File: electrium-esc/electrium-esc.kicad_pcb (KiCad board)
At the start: 2 copper layers, 90 x 60 mm, 181 parts, among them J1 Debug Connector, J2 USB_MICRO, J4 SERVO, J5 Conn_01x04_Male, Q1 IRF3205, Q10 IRF3205, Q11 IRF3205, Q12 IRF3205, Q2 IRF3205, Q3 IRF3205, Q4 IRF3205, Q5 IRF3205, Q6 IRF3205, Q7 IRF3205, Q8 IRF3205, Q9 IRF3205, SW1 SW_SPDT, U1 STM32F407ZGT6, U2 DRV8301DCAR, U3 DRV8301DCAR, U5 NRF24L01_Breakout, Y1 25MHz

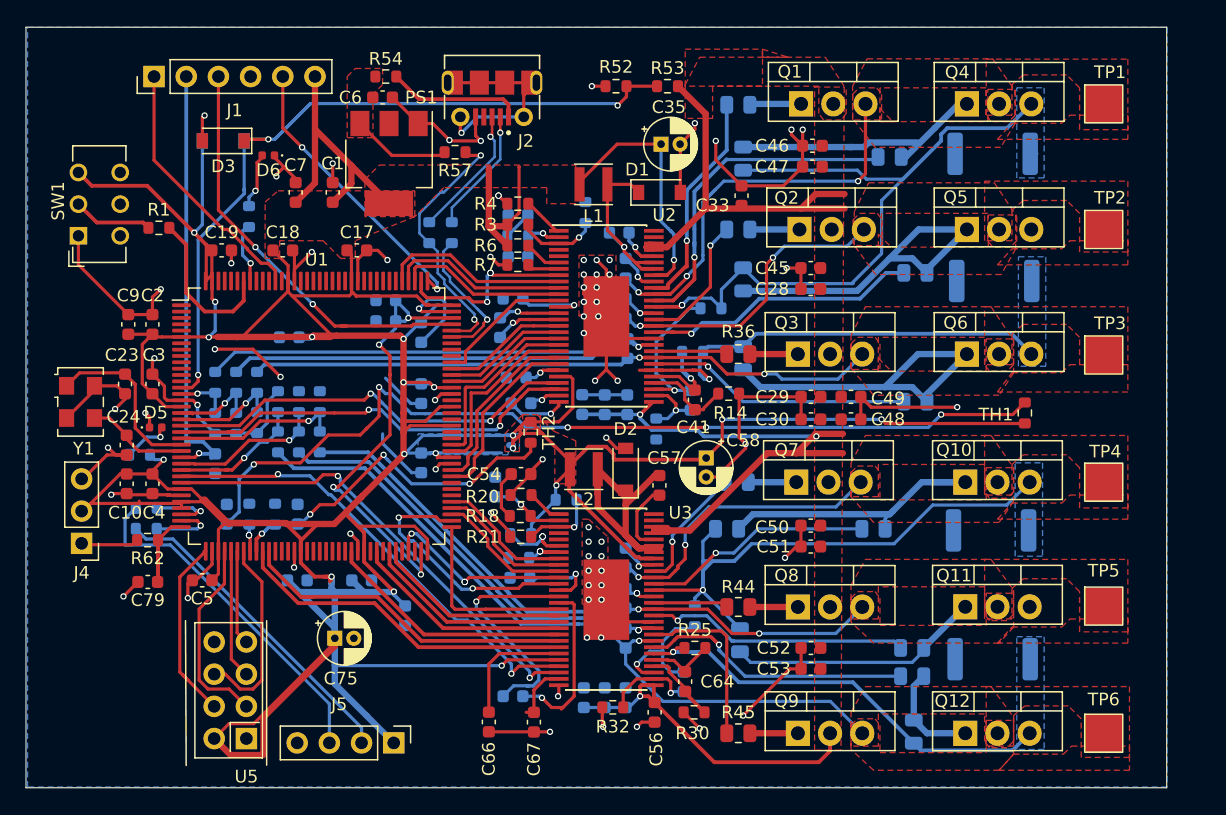
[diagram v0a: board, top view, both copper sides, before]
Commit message: Fix warnings
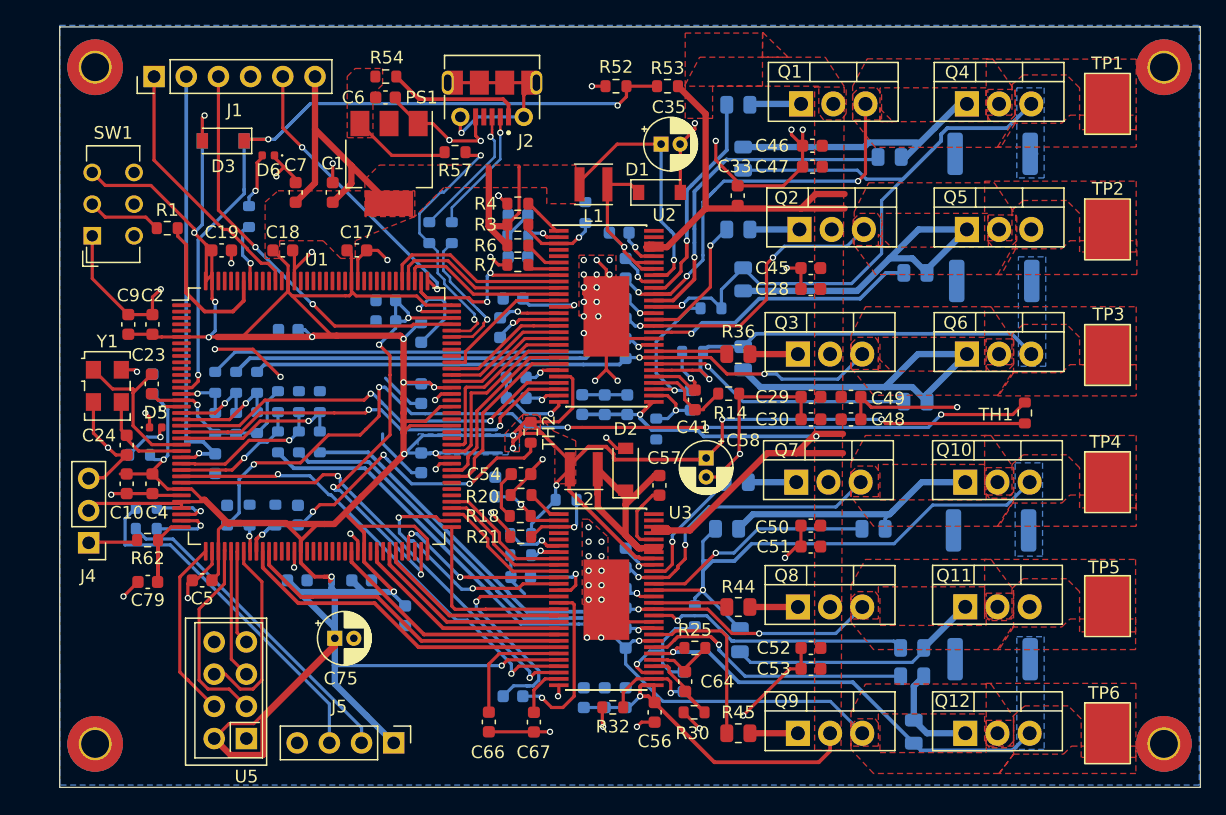
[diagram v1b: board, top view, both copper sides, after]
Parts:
- added REF**: MountingHole_2.2mm_M2_Pad_TopBottom, MountingHole:MountingHole_2.2mm_M2_Pad_TopBottom, F.Cu at (190.8, 102.1)
- added REF**: MountingHole_2.2mm_M2_Pad_TopBottom, MountingHole:MountingHole_2.2mm_M2_Pad_TopBottom, F.Cu at (106.5, 48.7)
- added REF**: MountingHole_2.2mm_M2_Pad_TopBottom, MountingHole:MountingHole_2.2mm_M2_Pad_TopBottom, F.Cu at (190.8, 48.7)
- added asd: MountingHole_2.2mm_M2_Pad_TopBottom, MountingHole:MountingHole_2.2mm_M2_Pad_TopBottom, F.Cu at (106.5, 102.1)
- C3: moved to B.Cu
- moved Y1 2.47 mm to (107.4, 73.8)
- moved C23 2.11 mm to (110.9, 73.7)
- moved SW1 1.09 mm to (106.2, 62.0)
- moved R1 0.66 mm to (112.2, 61.4)
- moved C8 0.59 mm to (121.7, 69.4)
- moved J4 0.56 mm to (106.0, 86.2)
- moved C44 0.56 mm to (139.7, 74.8)
- moved C33 0.30 mm to (157.2, 58.8)
- moved R23 0.25 mm to (140.1, 87.2)
- moved C6 0.23 mm to (129.4, 51.1)
- moved C40 0.15 mm to (148.3, 70.9)
- moved C60 0.08 mm to (140.1, 88.9)
- moved C76 0.08 mm to (116.9, 84.0)
- moved C77 0.08 mm to (122.5, 84.0)
- moved R71 0.08 mm to (118.7, 84.0)
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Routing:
- net +3.3V: track 437.8 -> 421.0 mm, vias 19 -> 20
- net GND: track 240.6 -> 236.0 mm, vias 74 -> 73
- net Net-(Q10-Pad1): track 23.8 -> 20.7 mm
- net Net-(C41-Pad1): track 9.63 -> 7.30 mm
- net /MCU (STM32F407ZGT6)/SCK_B: track 16.5 -> 14.5 mm, vias 3 -> 2
- net /Motor Driver B (DRV8301)/H3_VS: track 60.9 -> 59.0 mm
- net /MCU (STM32F407ZGT6)/BR_SO2_A: track 34.7 -> 32.8 mm
- net /Motor Driver A (DRV8301)/H1_VS: track 72.8 -> 71.2 mm
- net /MCU (STM32F407ZGT6)/H3_A: track 15.7 -> 14.2 mm
- net /Motor Driver B (DRV8301)/GVDD: track 7.58 -> 6.06 mm
- net /Motor Driver B (DRV8301)/DTC: track 5.24 -> 3.89 mm, vias 2 -> 1
- net /MCU (STM32F407ZGT6)/BR_SO1_A: track 34.6 -> 33.3 mm
- net /Motor Driver A (DRV8301)/H3_LOW: track 36.0 -> 34.8 mm
- net /Motor Driver A (DRV8301)/M_H1: track 18.5 -> 17.3 mm
- net /MCU (STM32F407ZGT6)/BR_SO1_B: track 38.1 -> 37.1 mm
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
